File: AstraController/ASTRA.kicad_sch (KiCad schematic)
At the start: 37 parts, among them J1 RJ45 (NEMA 17), J2 RJ45 (NEMA 17), J3 RJ45 (BNO085), J4 RJ45 (BNO085), J5 USB_A, P1 12V-DC, SW1 TOP, SW2 BOTTOM, SW3 LEFT, SW4 RIGHT, SW5 SELECT, SW6 RETURN, SW7 RESET, T1 TMC2209, T2 TMC2209, U1 MCP23017x-x-SP

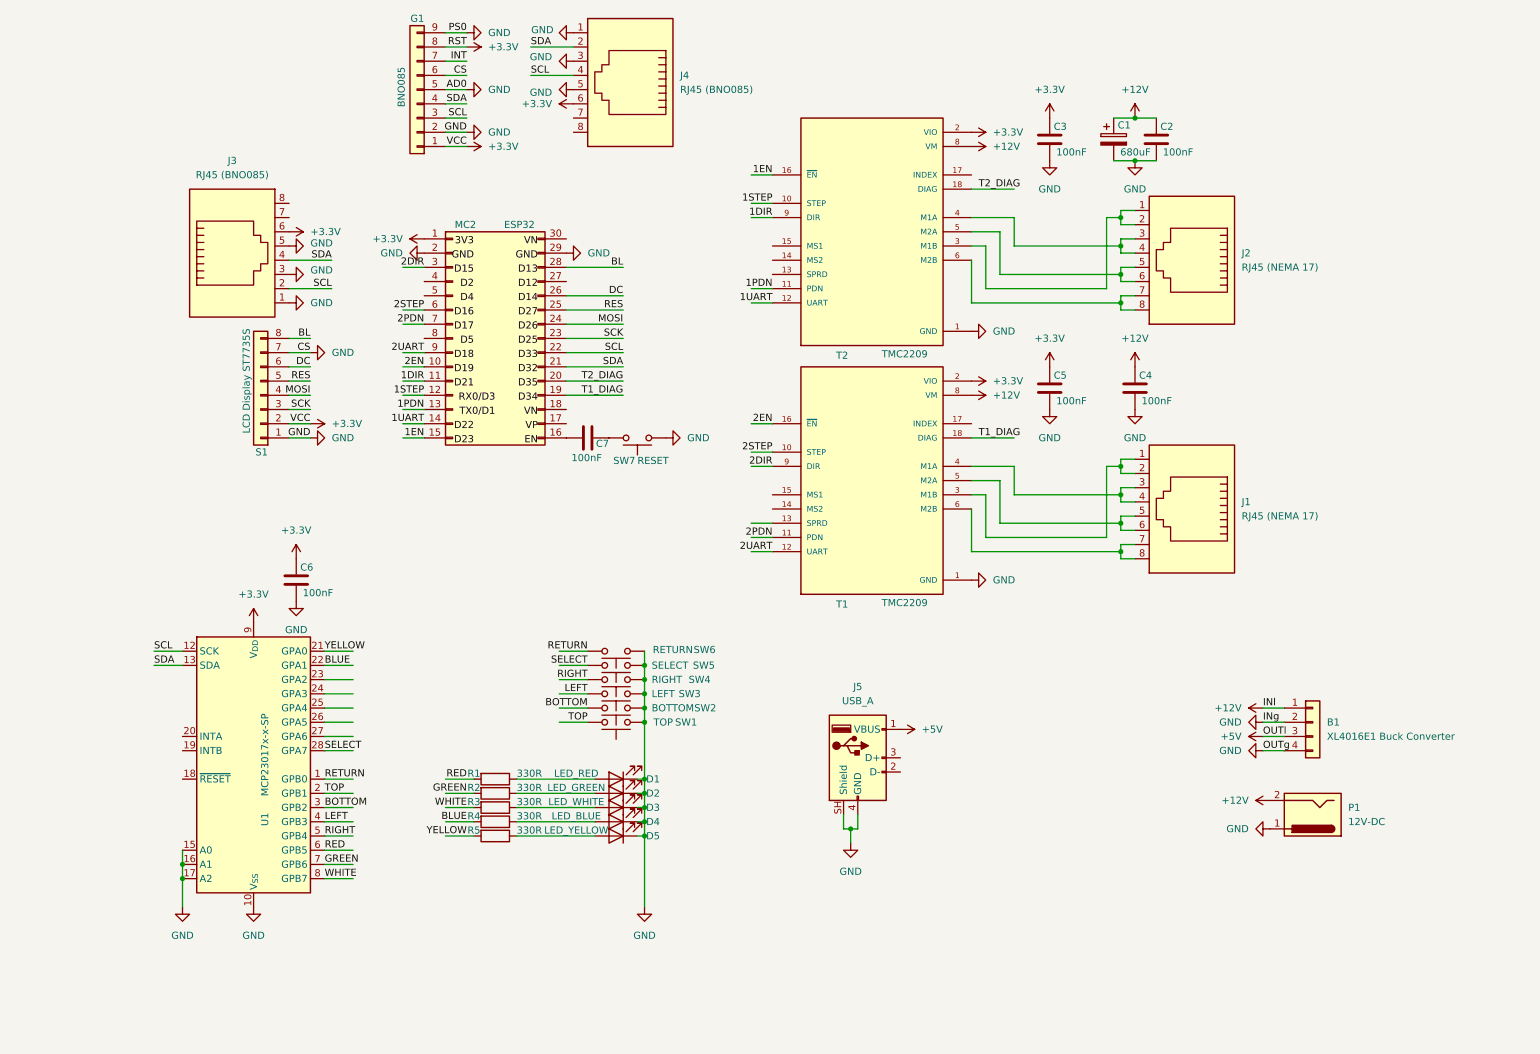
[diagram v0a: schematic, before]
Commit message: Ver 5
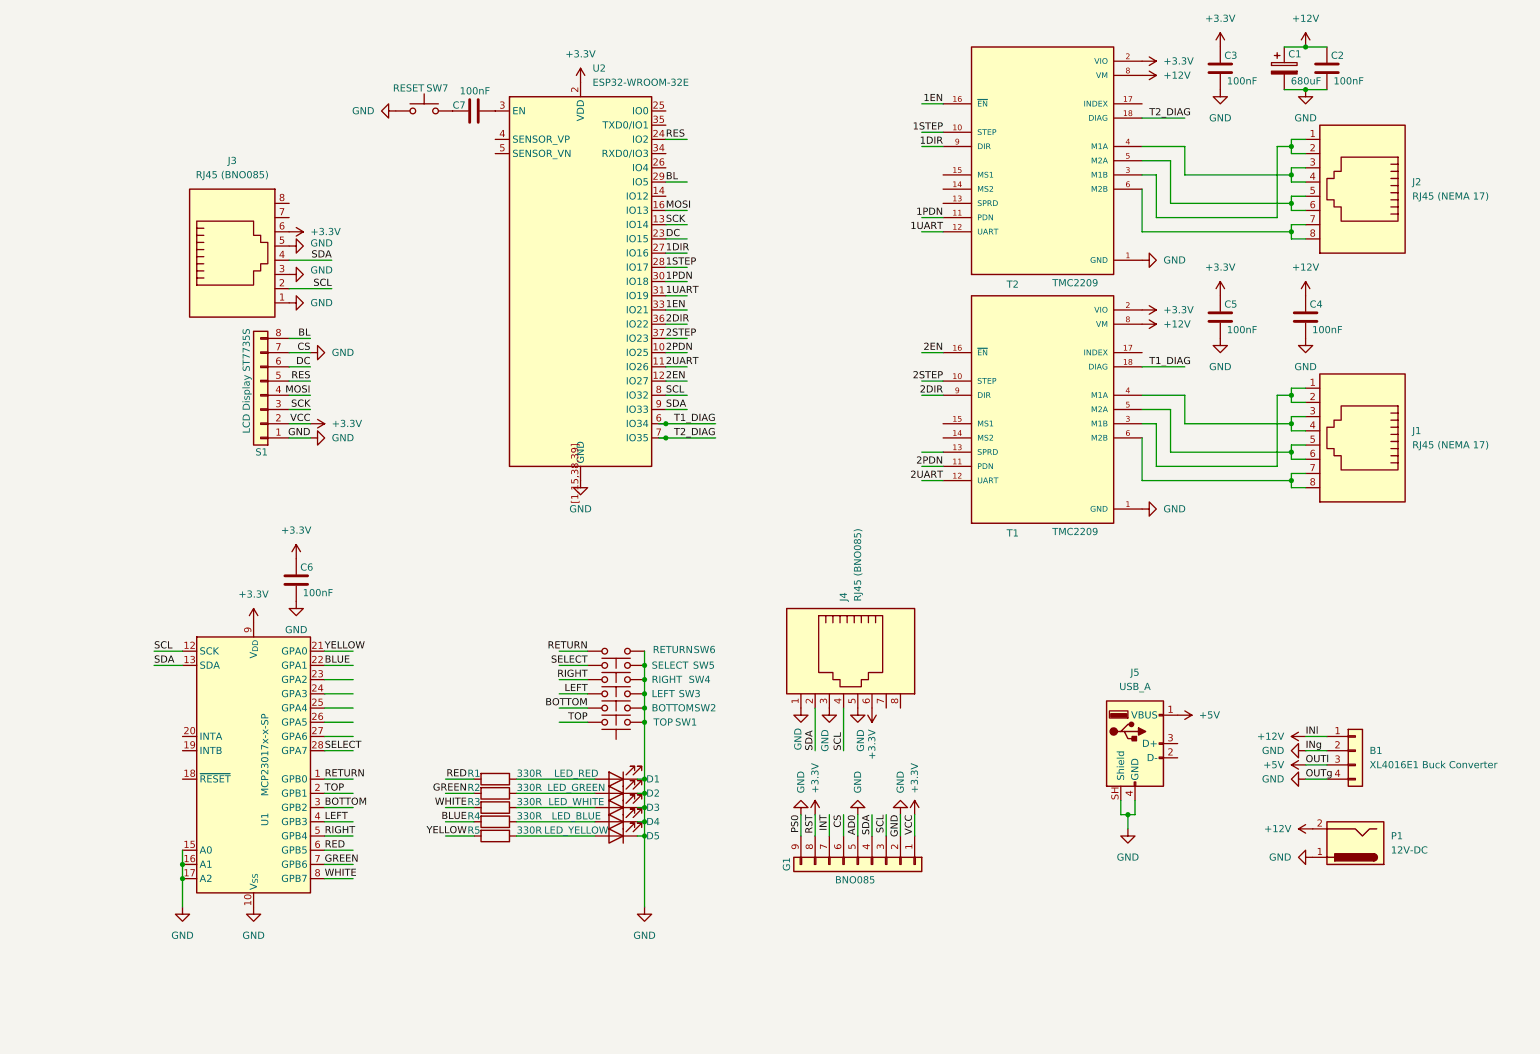
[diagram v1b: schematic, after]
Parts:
- removed MC2: ESP32, ASTRAfootprints:ESP32-WROOM-32D-Devkit, symbol Connector_Generic:Conn_02x15_Odd_Even
- added U2: ESP32-WROOM-32E, RF_Module:ESP32-WROOM-32E, symbol RF_Module:ESP32-WROOM-32E
- B1: footprint Connector_PinSocket_2.54mm:PinSocket_1x04_P2.54mm_Vertical -> TerminalBlock:TerminalBlock_MaiXu_MX126-5.0-04P_1x04_P5.00mm
- P1: footprint Connector_PinSocket_2.54mm:PinSocket_1x03_P2.54mm_Vertical -> TerminalBlock:TerminalBlock_MaiXu_MX126-5.0-02P_1x02_P5.00mm
- SW1, SW2, SW3, SW4, SW5, SW6, SW7: footprint Connector_PinSocket_2.54mm:PinSocket_1x02_P2.54mm_Vertical -> TerminalBlock:TerminalBlock_MaiXu_MX126-5.0-02P_1x02_P5.00mm
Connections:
- net +3.3V: now also U2.2 (VDD)
- net 1DIR: now also U2.27 (IO16)
- net 1EN: now also U2.33 (IO21)
- net 1PDN: now also U2.30 (IO18)
- net 1STEP: now also U2.28 (IO17)
- net 1UART: now also U2.31 (IO19)
- net 2DIR: now also U2.36 (IO22)
- net 2EN: now also U2.12 (IO27)
- net 2PDN: now also U2.10 (IO25)
- net 2STEP: now also U2.37 (IO23)
- net 2UART: now also U2.11 (IO26)
- net BL: now also U2.29 (IO5)
- net DC: now also U2.23 (IO15)
- net GND: now also U2.[1,15,38,39] (GND)
- net MOSI: now also U2.16 (IO13)
- net RES: now also U2.24 (IO2)
- net SCK: now also U2.13 (IO14)
- net SCL: now also U2.8 (IO32)
- net SDA: now also U2.9 (IO33)
- net T1_DIAG: now also U2.6 (IO34)
- net T2_DIAG: now also U2.7 (IO35)
- net at C7.2: now also U2.3 (EN)
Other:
- moved on the sheet: B1, C1, C2, C3, C4, C5, G1, J1, J2, J4, J5, P1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

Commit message: ver 5
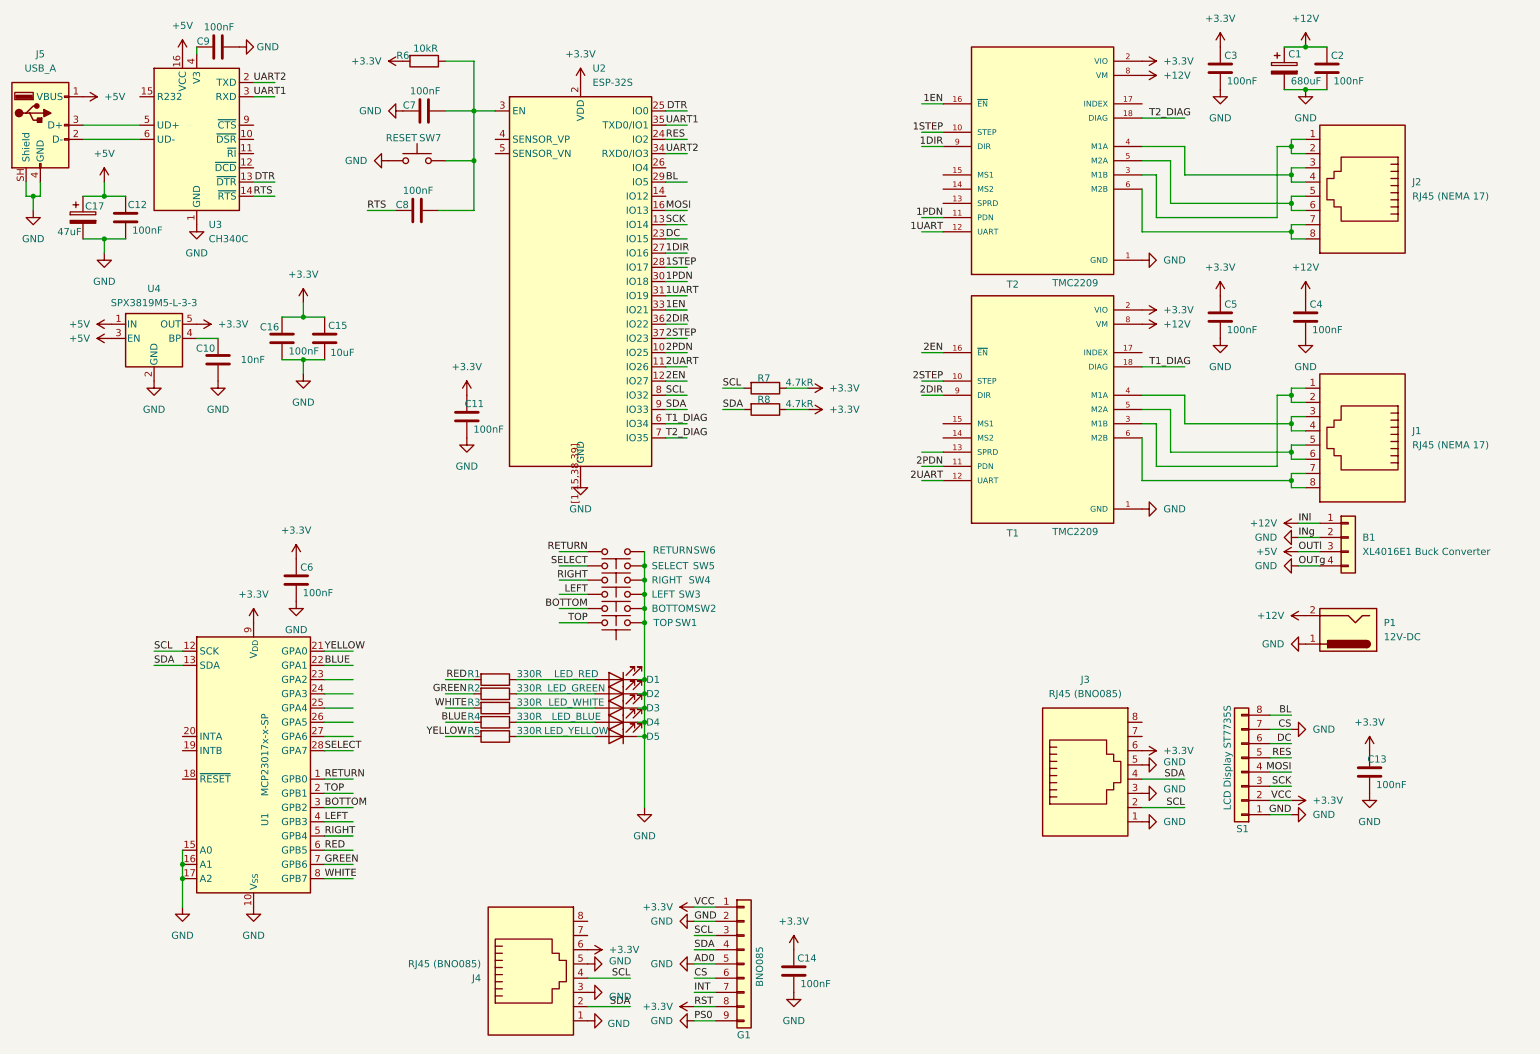
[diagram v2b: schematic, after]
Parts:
- added C10: 10nF, Capacitor_SMD:C_0805_2012Metric_Pad1.18x1.45mm_HandSolder, symbol Device:C
- added C11, C12, C13, C14, C16, C8, C9: 100nF, Capacitor_SMD:C_0805_2012Metric_Pad1.18x1.45mm_HandSolder, symbol Device:C
- added C15: 10uF, Capacitor_SMD:C_0805_2012Metric_Pad1.18x1.45mm_HandSolder, symbol Device:C
- added C17: 47uF, Capacitor_THT:CP_Radial_D10.0mm_P5.00mm, symbol Device:C_Polarized
- added R6: 10kR, Resistor_SMD:R_0805_2012Metric_Pad1.20x1.40mm_HandSolder, symbol Device:R
- added R7, R8: 4.7kR, Resistor_SMD:R_0805_2012Metric_Pad1.20x1.40mm_HandSolder, symbol Device:R
- added U3: CH340C, Package_SO:SOIC-16_3.9x9.9mm_P1.27mm, symbol Interface_USB:CH340C
- added U4: SPX3819M5-L-3-3, Package_TO_SOT_SMD:SOT-23-5, symbol Regulator_Linear:SPX3819M5-L-3-3
- B1: footprint TerminalBlock:TerminalBlock_MaiXu_MX126-5.0-04P_1x04_P5.00mm -> ASTRAfootprints:Double 1x02 screw connector
- P1, SW1, SW2, SW3, SW4, SW5, SW6, SW7: footprint TerminalBlock:TerminalBlock_MaiXu_MX126-5.0-02P_1x02_P5.00mm -> TerminalBlock:TerminalBlock_Xinya_XY308-2.54-2P_1x02_P2.54mm_Horizontal
- S1: footprint Connector_PinSocket_2.54mm:PinSocket_1x08_P2.54mm_Vertical -> ASTRAfootprints:Quadruple 1x02 screw connector
- U2: value ESP32-WROOM-32E -> ESP-32S
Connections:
- net +3.3V: now also C11.1, C13.1, C14.1, C15.1, C16.1, R6.2, R7.1, R8.1, U4.5 (OUT)
- net +5V: now also C12.1, C17.1, U3.16 (VCC), U4.1 (IN), U4.3 (EN)
- net GND: now also C7.1, C10.2, C11.2, C12.2, C13.2, C14.2, C15.2, C16.2, C17.2, C9.2, U3.1 (GND), U4.2 (GND)
- net SCL: now also R7.2
- net SDA: now also R8.2
- net at SW7.2: now also C7.2, U2.3 (EN), C8.2, R6.1; no longer C7.1
- net at J5.2 (D-): now also U3.6 (UD-)
- net at J5.3 (D+): now also U3.5 (UD+)
- net DTR: now reaches U2.25 (IO0)
- net DTR: now also U3.13 (~{DTR})
- net UART2: now reaches U2.34 (RXD0/IO3)
- net UART2: now also U3.2 (TXD)
- net UART1: now reaches U2.35 (TXD0/IO1)
- net UART1: now also U3.3 (RXD)
- new net: C10.1, U4.4 (BP)
- new net: C9.1, U3.4 (V3)
- new net RTS: C8.1, U3.14 (~{RTS})
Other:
- moved on the sheet: B1, C7, D1, D2, D3, D4, D5, G1, J3, J4, J5, P1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
